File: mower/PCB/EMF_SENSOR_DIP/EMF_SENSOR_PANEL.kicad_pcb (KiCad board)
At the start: 2 copper layers, 245 x 163 mm, 360 parts, among them J1 Conn_01x03_Pin, U1 LM358

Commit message: .
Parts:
- removed the C1 at (81.6, 151.0)
- removed the C1 at (40.6, 28.0)
- removed the C1 at (245.6, 28.0)
- removed the C1 at (122.6, 110.0)
- removed the C1 at (163.6, 110.0)
- removed the C1 at (40.6, 69.0)
- removed the C1 at (163.6, 69.0)
- removed the C1 at (40.6, 151.0)
- removed the C1 at (81.6, 69.0)
- removed the C1 at (163.6, 28.0)
- removed the C1 at (204.6, 110.0)
- removed the C1 at (122.6, 151.0)
- removed the C1 at (81.6, 28.0)
- removed the C1 at (245.6, 69.0)
- removed the C1 at (122.6, 69.0)
- removed the C1 at (81.6, 110.0)
- removed the C1 at (122.6, 28.0)
- removed the C1 at (204.6, 28.0)
- removed the C1 at (204.6, 151.0)
- removed the C1 at (245.6, 151.0)
- removed the C1 at (40.6, 110.0)
- removed the C1 at (204.6, 69.0)
- removed the C1 at (163.6, 151.0)
- removed the C1 at (245.6, 110.0)
- removed the C3 at (143.8, 106.8)
- removed the C3 at (225.8, 24.8)
- removed the C3 at (266.8, 106.8)
- removed the C3 at (61.8, 24.8)
- removed the C3 at (102.8, 106.8)
- removed the C3 at (225.8, 147.8)
- removed the C3 at (143.8, 65.8)
- removed the C3 at (61.8, 147.8)
- removed the C3 at (225.8, 65.8)
- removed the C3 at (102.8, 147.8)
- removed the C3 at (184.8, 65.8)
- removed the C3 at (266.8, 65.8)
- removed the C3 at (143.8, 24.8)
- removed the C3 at (266.8, 24.8)
- removed the C3 at (225.8, 106.8)
- removed the C3 at (143.8, 147.8)
- removed the C3 at (102.8, 65.8)
- removed the C3 at (184.8, 106.8)
- removed the C3 at (266.8, 147.8)
- removed the C3 at (102.8, 24.8)
- removed the C3 at (61.8, 106.8)
- removed the C3 at (61.8, 65.8)
- removed the C3 at (184.8, 147.8)
- removed the C3 at (184.8, 24.8)
- removed the D1 at (215.1, 82.0)
- removed the D1 at (51.1, 82.0)
- removed the D1 at (256.1, 123.0)
- removed the D1 at (215.1, 41.0)
- removed the D1 at (256.1, 82.0)
- removed the D1 at (133.1, 41.0)
- removed the D1 at (133.1, 123.0)
- removed the D1 at (174.1, 82.0)
- removed the D1 at (215.1, 164.0)
- removed the D1 at (51.1, 164.0)
- removed the D1 at (215.1, 123.0)
- removed the D1 at (92.1, 164.0)
- removed the D1 at (256.1, 41.0)
- removed the D1 at (174.1, 41.0)
- removed the D1 at (133.1, 164.0)
- removed the D1 at (51.1, 41.0)
- removed the D1 at (51.1, 123.0)
- removed the D1 at (92.1, 41.0)
- removed the D1 at (133.1, 82.0)
- removed the D1 at (92.1, 123.0)
- removed the D1 at (174.1, 164.0)
- removed the D1 at (174.1, 123.0)
- removed the D1 at (256.1, 164.0)
- removed the D1 at (92.1, 82.0)
- removed the D2 at (225.7, 167.2)
- removed the D2 at (61.7, 167.2)
- removed the D2 at (266.7, 44.2)
- removed the D2 at (102.7, 44.2)
- removed the D2 at (143.7, 44.2)
- removed the D2 at (225.7, 126.2)
- removed the D2 at (184.7, 44.2)
- removed the D2 at (266.7, 85.2)
- removed the D2 at (61.7, 44.2)
- removed the D2 at (102.7, 85.2)
- removed the D2 at (61.7, 126.2)
- removed the D2 at (266.7, 126.2)
- removed the D2 at (225.7, 44.2)
- removed the D2 at (102.7, 167.2)
- removed the D2 at (61.7, 85.2)
- removed the D2 at (184.7, 126.2)
- removed the D2 at (184.7, 167.2)
- removed the D2 at (266.7, 167.2)
- removed the D2 at (143.7, 85.2)
- removed the D2 at (143.7, 167.2)
- removed the D2 at (184.7, 85.2)
- removed the D2 at (225.7, 85.2)
- removed the D2 at (143.7, 126.2)
- removed the D2 at (102.7, 126.2)
- removed the J1 at (93.4, 148.4)
- removed the J1 at (257.4, 148.4)
- removed the J1 at (175.4, 66.4)
- removed the J1 at (216.4, 66.4)
- removed the J1 at (257.4, 25.4)
- removed the J1 at (134.4, 66.4)
- removed the J1 at (257.4, 66.4)
- removed the J1 at (93.4, 107.4)
- removed the J1 at (93.4, 66.4)
- removed the J1 at (134.4, 148.4)
- removed the J1 at (216.4, 107.4)
- removed the J1 at (257.4, 107.4)
- removed the J1 at (175.4, 25.4)
- removed the J1 at (52.4, 107.4)
- removed the J1 at (175.4, 107.4)
- removed the J1 at (216.4, 25.4)
- removed the J1 at (52.4, 66.4)
- removed the J1 at (93.4, 25.4)
- removed the J1 at (52.4, 25.4)
- removed the J1 at (134.4, 107.4)
- removed the J1 at (52.4, 148.4)
- removed the J1 at (134.4, 25.4)
- removed the J1 at (175.4, 148.4)
- removed the J1 at (216.4, 148.4)
- removed the L1 at (235.4, 54.8)
- removed the L1 at (30.4, 54.8)
- removed the L1 at (71.4, 136.8)
- removed the L1 at (112.4, 136.8)
- removed the L1 at (153.4, 177.8)
- removed the L1 at (194.4, 177.8)
- removed the L1 at (30.4, 95.8)
- removed the L1 at (71.4, 95.8)
- removed the L1 at (235.4, 177.8)
- removed the L1 at (194.4, 95.8)
- removed the L1 at (30.4, 177.8)
- removed the L1 at (30.4, 136.8)
- removed the L1 at (153.4, 136.8)
- removed the L1 at (235.4, 136.8)
- removed the L1 at (153.4, 95.8)
- removed the L1 at (71.4, 54.8)
- removed the L1 at (153.4, 54.8)
- removed the L1 at (112.4, 54.8)
- removed the L1 at (112.4, 95.8)
- removed the L1 at (112.4, 177.8)
- removed the L1 at (194.4, 136.8)
- removed the L1 at (71.4, 177.8)
- removed the L1 at (235.4, 95.8)
- removed the L1 at (194.4, 54.8)
- removed the R1 at (49.9, 174.4)
- removed the R1 at (254.9, 51.4)
- removed the R1 at (172.9, 92.4)
- removed the R1 at (213.9, 174.4)
- removed the R1 at (172.9, 51.4)
- removed the R1 at (131.9, 133.4)
- removed the R1 at (90.9, 51.4)
- removed the R1 at (254.9, 133.4)
- removed the R1 at (90.9, 174.4)
- removed the R1 at (254.9, 92.4)
- removed the R1 at (172.9, 133.4)
- removed the R1 at (254.9, 174.4)
- removed the R1 at (49.9, 133.4)
- removed the R1 at (49.9, 92.4)
- removed the R1 at (90.9, 92.4)
- removed the R1 at (213.9, 51.4)
- removed the R1 at (131.9, 92.4)
- removed the R1 at (90.9, 133.4)
- removed the R1 at (49.9, 51.4)
- removed the R1 at (213.9, 133.4)
- removed the R1 at (172.9, 174.4)
- removed the R1 at (213.9, 92.4)
- removed the R1 at (131.9, 51.4)
- removed the R1 at (131.9, 174.4)
- removed the R2 at (215.3, 154.2)
- removed the R2 at (133.3, 31.2)
- removed the R2 at (51.3, 113.2)
- removed the R2 at (256.3, 72.2)
- removed the R2 at (174.3, 154.2)
- removed the R2 at (215.3, 113.2)
- removed the R2 at (215.3, 31.2)
- removed the R2 at (256.3, 31.2)
- removed the R2 at (133.3, 154.2)
- removed the R2 at (256.3, 113.2)
- removed the R2 at (92.3, 154.2)
- removed the R2 at (133.3, 113.2)
- removed the R2 at (92.3, 113.2)
- removed the R2 at (51.3, 72.2)
- removed the R2 at (256.3, 154.2)
- removed the R2 at (92.3, 72.2)
- removed the R2 at (51.3, 154.2)
- removed the R2 at (174.3, 113.2)
- removed the R2 at (215.3, 72.2)
- removed the R2 at (92.3, 31.2)
- removed the R2 at (133.3, 72.2)
- removed the R2 at (174.3, 72.2)
- removed the R2 at (51.3, 31.2)
- removed the R2 at (174.3, 31.2)
- removed the R3 at (197.2, 130.9)
- removed the R3 at (238.2, 171.9)
- removed the R3 at (197.2, 48.9)
- removed the R3 at (33.2, 130.9)
- removed the R3 at (115.2, 48.9)
- removed the R3 at (74.2, 89.9)
- removed the R3 at (115.2, 171.9)
- removed the R3 at (238.2, 89.9)
- removed the R3 at (156.2, 130.9)
- removed the R3 at (197.2, 89.9)
- removed the R3 at (33.2, 48.9)
- removed the R3 at (238.2, 130.9)
- removed the R3 at (33.2, 89.9)
- removed the R3 at (156.2, 89.9)
- removed the R3 at (115.2, 89.9)
- removed the R3 at (74.2, 171.9)
- removed the R3 at (197.2, 171.9)
- removed the R3 at (238.2, 48.9)
- removed the R3 at (74.2, 130.9)
- removed the R3 at (156.2, 171.9)
- removed the R3 at (156.2, 48.9)
- removed the R3 at (74.2, 48.9)
- removed the R3 at (115.2, 130.9)
- removed the R3 at (33.2, 171.9)
- removed the R4 at (200.6, 38.9)
- removed the R4 at (36.6, 161.9)
- removed the R4 at (36.6, 79.9)
- removed the R4 at (159.6, 161.9)
- removed the R4 at (118.6, 79.9)
- removed the R4 at (200.6, 161.9)
- removed the R4 at (36.6, 120.9)
- removed the R4 at (118.6, 38.9)
- removed the R4 at (118.6, 161.9)
- removed the R4 at (77.6, 161.9)
- removed the R4 at (36.6, 38.9)
- removed the R4 at (159.6, 79.9)
- removed the R4 at (241.6, 161.9)
- removed the R4 at (241.6, 79.9)
- removed the R4 at (200.6, 120.9)
- removed the R4 at (159.6, 120.9)
- removed the R4 at (118.6, 120.9)
- removed the R4 at (77.6, 120.9)
- removed the R4 at (200.6, 79.9)
- removed the R4 at (77.6, 38.9)
- removed the R4 at (241.6, 38.9)
- removed the R4 at (77.6, 79.9)
- removed the R4 at (159.6, 38.9)
- removed the R4 at (241.6, 120.9)
- removed the R5 at (77.2, 51.7)
- removed the R5 at (200.2, 174.7)
- removed the R5 at (159.2, 51.7)
- removed the R5 at (241.2, 174.7)
- removed the R5 at (241.2, 51.7)
- removed the R5 at (77.2, 92.7)
- removed the R5 at (118.2, 92.7)
- removed the R5 at (200.2, 51.7)
- removed the R5 at (118.2, 174.7)
- removed the R5 at (200.2, 133.7)
- removed the R5 at (118.2, 133.7)
- removed the R5 at (77.2, 133.7)
- removed the R5 at (159.2, 133.7)
- removed the R5 at (159.2, 174.7)
- removed the R5 at (200.2, 92.7)
- removed the R5 at (241.2, 133.7)
- removed the R5 at (159.2, 92.7)
- removed the R5 at (118.2, 51.7)
- removed the R5 at (36.2, 133.7)
- removed the R5 at (36.2, 51.7)
- removed the R5 at (77.2, 174.7)
- removed the R5 at (36.2, 92.7)
- removed the R5 at (241.2, 92.7)
- removed the R5 at (36.2, 174.7)
- removed the R6 at (61.9, 34.4)
- removed the R6 at (143.9, 75.4)
- removed the R6 at (102.9, 75.4)
- removed the R6 at (266.9, 75.4)
- removed the R6 at (61.9, 157.4)
- removed the R6 at (266.9, 157.4)
- removed the R6 at (266.9, 116.4)
- removed the R6 at (102.9, 157.4)
- removed the R6 at (184.9, 34.4)
- removed the R6 at (143.9, 116.4)
- removed the R6 at (61.9, 116.4)
- removed the R6 at (102.9, 116.4)
- removed the R6 at (266.9, 34.4)
- removed the R6 at (225.9, 116.4)
- removed the R6 at (225.9, 75.4)
- removed the R6 at (143.9, 34.4)
- removed the R6 at (102.9, 34.4)
- removed the R6 at (184.9, 157.4)
- removed the R6 at (184.9, 75.4)
- removed the R6 at (225.9, 34.4)
- removed the R6 at (143.9, 157.4)
- removed the R6 at (61.9, 75.4)
- removed the R6 at (225.9, 157.4)
- removed the R6 at (184.9, 116.4)
- removed the R7 at (174.7, 170.6)
- removed the R7 at (215.7, 170.6)
- removed the R7 at (51.7, 170.6)
- removed the R7 at (92.7, 47.6)
- removed the R7 at (256.7, 170.6)
- removed the R7 at (256.7, 129.6)
- removed the R7 at (215.7, 47.6)
- removed the R7 at (133.7, 47.6)
- removed the R7 at (92.7, 129.6)
- removed the R7 at (256.7, 88.6)
- removed the R7 at (51.7, 88.6)
- removed the R7 at (133.7, 88.6)
- removed the R7 at (133.7, 170.6)
- removed the R7 at (174.7, 129.6)
- removed the R7 at (256.7, 47.6)
- removed the R7 at (174.7, 88.6)
- removed the R7 at (133.7, 129.6)
- removed the R7 at (215.7, 129.6)
- removed the R7 at (215.7, 88.6)
- removed the R7 at (92.7, 88.6)
- removed the R7 at (92.7, 170.6)
- removed the R7 at (174.7, 47.6)
- removed the R7 at (51.7, 47.6)
- removed the R7 at (51.7, 129.6)
- removed the R9 at (185.0, 160.8)
- removed the R9 at (226.0, 37.8)
- removed the R9 at (144.0, 160.8)
- removed the R9 at (103.0, 37.8)
- removed the R9 at (103.0, 119.8)
- removed the R9 at (185.0, 78.8)
- removed the R9 at (144.0, 119.8)
- removed the R9 at (185.0, 119.8)
- removed the R9 at (103.0, 78.8)
- removed the R9 at (62.0, 160.8)
- removed the R9 at (267.0, 160.8)
- removed the R9 at (62.0, 119.8)
- removed the R9 at (226.0, 160.8)
- removed the R9 at (267.0, 37.8)
- removed the R9 at (62.0, 78.8)
- removed the R9 at (185.0, 37.8)
- removed the R9 at (62.0, 37.8)
- removed the R9 at (267.0, 78.8)
- removed the R9 at (144.0, 37.8)
- removed the R9 at (103.0, 160.8)
- removed the R9 at (226.0, 78.8)
- removed the R9 at (226.0, 119.8)
- removed the R9 at (144.0, 78.8)
- removed the R9 at (267.0, 119.8)
- removed the U1 at (122.2, 35.2)
- removed the U1 at (81.2, 76.2)
- removed the U1 at (81.2, 35.2)
- removed the U1 at (122.2, 117.2)
- removed the U1 at (204.2, 76.2)
- removed the U1 at (81.2, 117.2)
- removed the U1 at (122.2, 76.2)
- removed the U1 at (163.2, 35.2)
- removed the U1 at (163.2, 158.2)
- removed the U1 at (163.2, 76.2)
- removed the U1 at (163.2, 117.2)
- removed the U1 at (245.2, 35.2)
- removed the U1 at (81.2, 158.2)
- removed the U1 at (122.2, 158.2)
- removed the U1 at (204.2, 158.2)
- removed the U1 at (204.2, 117.2)
- removed the U1 at (245.2, 76.2)
- removed the U1 at (245.2, 117.2)
- removed the U1 at (204.2, 35.2)
- removed the U1 at (40.2, 117.2)
- removed the U1 at (40.2, 76.2)
- removed the U1 at (245.2, 158.2)
- removed the U1 at (40.2, 158.2)
- removed the U1 at (40.2, 35.2)
- added C1: 100nF, IMRANS_LIBRARY:C_Disc_D3.0mm_W1.6mm_P2.50mm, F.Cu at (193.3, 105.8)
- added C1: 100nF, IMRANS_LIBRARY:C_Disc_D3.0mm_W1.6mm_P2.50mm, F.Cu at (42.5, 139.8)
- added C1: 100nF, IMRANS_LIBRARY:C_Disc_D3.0mm_W1.6mm_P2.50mm, F.Cu at (117.9, 105.8)
- added C1: 100nF, IMRANS_LIBRARY:C_Disc_D3.0mm_W1.6mm_P2.50mm, F.Cu at (42.5, 71.8)
- added C1: 100nF, IMRANS_LIBRARY:C_Disc_D3.0mm_W1.6mm_P2.50mm, F.Cu at (193.3, 37.8)
- added C1: 100nF, IMRANS_LIBRARY:C_Disc_D3.0mm_W1.6mm_P2.50mm, F.Cu at (193.3, 139.8)
- added C1: 100nF, IMRANS_LIBRARY:C_Disc_D3.0mm_W1.6mm_P2.50mm, F.Cu at (117.9, 37.8)
- added C1: 100nF, IMRANS_LIBRARY:C_Disc_D3.0mm_W1.6mm_P2.50mm, F.Cu at (117.9, 139.8)
- added C1: 100nF, IMRANS_LIBRARY:C_Disc_D3.0mm_W1.6mm_P2.50mm, F.Cu at (42.5, 105.8)
- added C1: 100nF, IMRANS_LIBRARY:C_Disc_D3.0mm_W1.6mm_P2.50mm, F.Cu at (117.9, 71.8)
- added C1: 100nF, IMRANS_LIBRARY:C_Disc_D3.0mm_W1.6mm_P2.50mm, F.Cu at (42.5, 37.8)
- added C1: 100nF, IMRANS_LIBRARY:C_Disc_D3.0mm_W1.6mm_P2.50mm, F.Cu at (193.3, 71.8)
- added C2: 10uF, IMRANS_LIBRARY:C_Disc_D3.0mm_W1.6mm_P2.50mm, F.Cu at (245.9, 149.2)
- added C2: 10uF, IMRANS_LIBRARY:C_Disc_D3.0mm_W1.6mm_P2.50mm, F.Cu at (170.5, 47.2)
- added C2: 10uF, IMRANS_LIBRARY:C_Disc_D3.0mm_W1.6mm_P2.50mm, F.Cu at (170.5, 149.2)
- added C2: 10uF, IMRANS_LIBRARY:C_Disc_D3.0mm_W1.6mm_P2.50mm, F.Cu at (170.5, 81.2)
- added C2: 10uF, IMRANS_LIBRARY:C_Disc_D3.0mm_W1.6mm_P2.50mm, F.Cu at (245.9, 47.2)
- added C2: 10uF, IMRANS_LIBRARY:C_Disc_D3.0mm_W1.6mm_P2.50mm, F.Cu at (245.9, 115.2)
- added C2: 10uF, IMRANS_LIBRARY:C_Disc_D3.0mm_W1.6mm_P2.50mm, F.Cu at (95.1, 47.2)
- added C2: 10uF, IMRANS_LIBRARY:C_Disc_D3.0mm_W1.6mm_P2.50mm, F.Cu at (170.5, 115.2)
- added C2: 10uF, IMRANS_LIBRARY:C_Disc_D3.0mm_W1.6mm_P2.50mm, F.Cu at (95.1, 115.2)
- added C2: 10uF, IMRANS_LIBRARY:C_Disc_D3.0mm_W1.6mm_P2.50mm, F.Cu at (245.9, 81.2)
- added C2: 10uF, IMRANS_LIBRARY:C_Disc_D3.0mm_W1.6mm_P2.50mm, F.Cu at (95.1, 149.2)
- added C2: 10uF, IMRANS_LIBRARY:C_Disc_D3.0mm_W1.6mm_P2.50mm, F.Cu at (95.1, 81.2)
- added C3: 100nF (104), IMRANS_LIBRARY:C_Disc_D3.0mm_W1.6mm_P2.50mm, F.Cu at (83.1, 43.8)
- added C3: 100nF (104), IMRANS_LIBRARY:C_Disc_D3.0mm_W1.6mm_P2.50mm, F.Cu at (233.9, 43.8)
- added C3: 100nF (104), IMRANS_LIBRARY:C_Disc_D3.0mm_W1.6mm_P2.50mm, F.Cu at (158.5, 145.8)
- added C3: 100nF (104), IMRANS_LIBRARY:C_Disc_D3.0mm_W1.6mm_P2.50mm, F.Cu at (83.1, 77.8)
- added C3: 100nF (104), IMRANS_LIBRARY:C_Disc_D3.0mm_W1.6mm_P2.50mm, F.Cu at (83.1, 111.8)
- added C3: 100nF (104), IMRANS_LIBRARY:C_Disc_D3.0mm_W1.6mm_P2.50mm, F.Cu at (158.5, 43.8)
- added C3: 100nF (104), IMRANS_LIBRARY:C_Disc_D3.0mm_W1.6mm_P2.50mm, F.Cu at (233.9, 77.8)
- added C3: 100nF (104), IMRANS_LIBRARY:C_Disc_D3.0mm_W1.6mm_P2.50mm, F.Cu at (158.5, 77.8)
- added C3: 100nF (104), IMRANS_LIBRARY:C_Disc_D3.0mm_W1.6mm_P2.50mm, F.Cu at (233.9, 111.8)
- added C3: 100nF (104), IMRANS_LIBRARY:C_Disc_D3.0mm_W1.6mm_P2.50mm, F.Cu at (233.9, 145.8)
- added C3: 100nF (104), IMRANS_LIBRARY:C_Disc_D3.0mm_W1.6mm_P2.50mm, F.Cu at (158.5, 111.8)
- added C3: 100nF (104), IMRANS_LIBRARY:C_Disc_D3.0mm_W1.6mm_P2.50mm, F.Cu at (83.1, 145.8)
- added C4: 10uF, IMRANS_LIBRARY:C_Disc_D3.0mm_W1.6mm_P2.50mm, F.Cu at (177.1, 60.4)
- added C4: 10uF, IMRANS_LIBRARY:C_Disc_D3.0mm_W1.6mm_P2.50mm, F.Cu at (101.7, 94.4)
- added C4: 10uF, IMRANS_LIBRARY:C_Disc_D3.0mm_W1.6mm_P2.50mm, F.Cu at (252.5, 26.4)
- added C4: 10uF, IMRANS_LIBRARY:C_Disc_D3.0mm_W1.6mm_P2.50mm, F.Cu at (252.5, 128.4)
- added C4: 10uF, IMRANS_LIBRARY:C_Disc_D3.0mm_W1.6mm_P2.50mm, F.Cu at (252.5, 94.4)
- added C4: 10uF, IMRANS_LIBRARY:C_Disc_D3.0mm_W1.6mm_P2.50mm, F.Cu at (101.7, 26.4)
- added C4: 10uF, IMRANS_LIBRARY:C_Disc_D3.0mm_W1.6mm_P2.50mm, F.Cu at (177.1, 128.4)
- added C4: 10uF, IMRANS_LIBRARY:C_Disc_D3.0mm_W1.6mm_P2.50mm, F.Cu at (177.1, 94.4)
- added C4: 10uF, IMRANS_LIBRARY:C_Disc_D3.0mm_W1.6mm_P2.50mm, F.Cu at (101.7, 128.4)
- added C4: 10uF, IMRANS_LIBRARY:C_Disc_D3.0mm_W1.6mm_P2.50mm, F.Cu at (101.7, 60.4)
- added C4: 10uF, IMRANS_LIBRARY:C_Disc_D3.0mm_W1.6mm_P2.50mm, F.Cu at (252.5, 60.4)
- added C4: 10uF, IMRANS_LIBRARY:C_Disc_D3.0mm_W1.6mm_P2.50mm, F.Cu at (177.1, 26.4)
- added C5: 1nF, IMRANS_LIBRARY:C_Disc_D3.0mm_W1.6mm_P2.50mm, F.Cu at (45.3, 29.8)
- added C5: 1nF, IMRANS_LIBRARY:C_Disc_D3.0mm_W1.6mm_P2.50mm, F.Cu at (45.3, 63.8)
- added C5: 1nF, IMRANS_LIBRARY:C_Disc_D3.0mm_W1.6mm_P2.50mm, F.Cu at (196.1, 131.8)
- added C5: 1nF, IMRANS_LIBRARY:C_Disc_D3.0mm_W1.6mm_P2.50mm, F.Cu at (120.7, 29.8)
- added C5: 1nF, IMRANS_LIBRARY:C_Disc_D3.0mm_W1.6mm_P2.50mm, F.Cu at (120.7, 97.8)
- added C5: 1nF, IMRANS_LIBRARY:C_Disc_D3.0mm_W1.6mm_P2.50mm, F.Cu at (45.3, 131.8)
- added C5: 1nF, IMRANS_LIBRARY:C_Disc_D3.0mm_W1.6mm_P2.50mm, F.Cu at (196.1, 97.8)
- added C5: 1nF, IMRANS_LIBRARY:C_Disc_D3.0mm_W1.6mm_P2.50mm, F.Cu at (196.1, 29.8)
- added C5: 1nF, IMRANS_LIBRARY:C_Disc_D3.0mm_W1.6mm_P2.50mm, F.Cu at (196.1, 63.8)
- added C5: 1nF, IMRANS_LIBRARY:C_Disc_D3.0mm_W1.6mm_P2.50mm, F.Cu at (120.7, 63.8)
- added C5: 1nF, IMRANS_LIBRARY:C_Disc_D3.0mm_W1.6mm_P2.50mm, F.Cu at (120.7, 131.8)
- added C5: 1nF, IMRANS_LIBRARY:C_Disc_D3.0mm_W1.6mm_P2.50mm, F.Cu at (45.3, 97.8)
- added C6: 0.01uF, IMRANS_LIBRARY:C_Disc_D3.0mm_W1.6mm_P2.50mm, F.Cu at (194.9, 125.2)
- added C6: 0.01uF, IMRANS_LIBRARY:C_Disc_D3.0mm_W1.6mm_P2.50mm, F.Cu at (194.9, 57.2)
- added C6: 0.01uF, IMRANS_LIBRARY:C_Disc_D3.0mm_W1.6mm_P2.50mm, F.Cu at (44.1, 91.2)
- added C6: 0.01uF, IMRANS_LIBRARY:C_Disc_D3.0mm_W1.6mm_P2.50mm, F.Cu at (194.9, 91.2)
- added C6: 0.01uF, IMRANS_LIBRARY:C_Disc_D3.0mm_W1.6mm_P2.50mm, F.Cu at (119.5, 125.2)
- added C6: 0.01uF, IMRANS_LIBRARY:C_Disc_D3.0mm_W1.6mm_P2.50mm, F.Cu at (119.5, 91.2)
- added C6: 0.01uF, IMRANS_LIBRARY:C_Disc_D3.0mm_W1.6mm_P2.50mm, F.Cu at (44.1, 57.2)
- added C6: 0.01uF, IMRANS_LIBRARY:C_Disc_D3.0mm_W1.6mm_P2.50mm, F.Cu at (119.5, 57.2)
- added C6: 0.01uF, IMRANS_LIBRARY:C_Disc_D3.0mm_W1.6mm_P2.50mm, F.Cu at (194.9, 23.2)
- added C6: 0.01uF, IMRANS_LIBRARY:C_Disc_D3.0mm_W1.6mm_P2.50mm, F.Cu at (44.1, 125.2)
- added C6: 0.01uF, IMRANS_LIBRARY:C_Disc_D3.0mm_W1.6mm_P2.50mm, F.Cu at (44.1, 23.2)
- added C6: 0.01uF, IMRANS_LIBRARY:C_Disc_D3.0mm_W1.6mm_P2.50mm, F.Cu at (119.5, 23.2)
- added D1: 1N4007, IMRANS_LIBRARY:R_Axial_DIN0207_L6.3mm_D2.5mm_P10.16mm_Horizontal_2, F.Cu at (159.2, 74.8)
- added D1: 1N4007, IMRANS_LIBRARY:R_Axial_DIN0207_L6.3mm_D2.5mm_P10.16mm_Horizontal_2, F.Cu at (83.8, 142.8)
- added D1: 1N4007, IMRANS_LIBRARY:R_Axial_DIN0207_L6.3mm_D2.5mm_P10.16mm_Horizontal_2, F.Cu at (159.2, 108.8)
- added D1: 1N4007, IMRANS_LIBRARY:R_Axial_DIN0207_L6.3mm_D2.5mm_P10.16mm_Horizontal_2, F.Cu at (83.8, 40.8)
- added D1: 1N4007, IMRANS_LIBRARY:R_Axial_DIN0207_L6.3mm_D2.5mm_P10.16mm_Horizontal_2, F.Cu at (83.8, 74.8)
- added D1: 1N4007, IMRANS_LIBRARY:R_Axial_DIN0207_L6.3mm_D2.5mm_P10.16mm_Horizontal_2, F.Cu at (159.2, 142.8)
- added D1: 1N4007, IMRANS_LIBRARY:R_Axial_DIN0207_L6.3mm_D2.5mm_P10.16mm_Horizontal_2, F.Cu at (234.6, 40.8)
- added D1: 1N4007, IMRANS_LIBRARY:R_Axial_DIN0207_L6.3mm_D2.5mm_P10.16mm_Horizontal_2, F.Cu at (83.8, 108.8)
- added D1: 1N4007, IMRANS_LIBRARY:R_Axial_DIN0207_L6.3mm_D2.5mm_P10.16mm_Horizontal_2, F.Cu at (234.6, 142.8)
- added D1: 1N4007, IMRANS_LIBRARY:R_Axial_DIN0207_L6.3mm_D2.5mm_P10.16mm_Horizontal_2, F.Cu at (159.2, 40.8)
- added D1: 1N4007, IMRANS_LIBRARY:R_Axial_DIN0207_L6.3mm_D2.5mm_P10.16mm_Horizontal_2, F.Cu at (234.6, 108.8)
- added D1: 1N4007, IMRANS_LIBRARY:R_Axial_DIN0207_L6.3mm_D2.5mm_P10.16mm_Horizontal_2, F.Cu at (234.6, 74.8)
- added D2: 1N5819, IMRANS_LIBRARY:R_Axial_DIN0207_L6.3mm_D2.5mm_P10.16mm_Horizontal_2, F.Cu at (223.8, 101.4)
- added D2: 1N5819, IMRANS_LIBRARY:R_Axial_DIN0207_L6.3mm_D2.5mm_P10.16mm_Horizontal_2, F.Cu at (148.4, 101.4)
- added D2: 1N5819, IMRANS_LIBRARY:R_Axial_DIN0207_L6.3mm_D2.5mm_P10.16mm_Horizontal_2, F.Cu at (73.0, 101.4)
- added D2: 1N5819, IMRANS_LIBRARY:R_Axial_DIN0207_L6.3mm_D2.5mm_P10.16mm_Horizontal_2, F.Cu at (223.8, 33.4)
- added D2: 1N5819, IMRANS_LIBRARY:R_Axial_DIN0207_L6.3mm_D2.5mm_P10.16mm_Horizontal_2, F.Cu at (223.8, 135.4)
- added D2: 1N5819, IMRANS_LIBRARY:R_Axial_DIN0207_L6.3mm_D2.5mm_P10.16mm_Horizontal_2, F.Cu at (73.0, 33.4)
- added D2: 1N5819, IMRANS_LIBRARY:R_Axial_DIN0207_L6.3mm_D2.5mm_P10.16mm_Horizontal_2, F.Cu at (148.4, 135.4)
- added D2: 1N5819, IMRANS_LIBRARY:R_Axial_DIN0207_L6.3mm_D2.5mm_P10.16mm_Horizontal_2, F.Cu at (223.8, 67.4)
- added D2: 1N5819, IMRANS_LIBRARY:R_Axial_DIN0207_L6.3mm_D2.5mm_P10.16mm_Horizontal_2, F.Cu at (148.4, 33.4)
- added D2: 1N5819, IMRANS_LIBRARY:R_Axial_DIN0207_L6.3mm_D2.5mm_P10.16mm_Horizontal_2, F.Cu at (73.0, 135.4)
- added D2: 1N5819, IMRANS_LIBRARY:R_Axial_DIN0207_L6.3mm_D2.5mm_P10.16mm_Horizontal_2, F.Cu at (148.4, 67.4)
- added D2: 1N5819, IMRANS_LIBRARY:R_Axial_DIN0207_L6.3mm_D2.5mm_P10.16mm_Horizontal_2, F.Cu at (73.0, 67.4)
- added J1: Conn_01x03_Pin, IMRANS_LIBRARY:PinHeader_1x03_P2.54mm_Vertical, F.Cu at (166.9, 61.4)
- added J1: Conn_01x03_Pin, IMRANS_LIBRARY:PinHeader_1x03_P2.54mm_Vertical, F.Cu at (166.9, 129.4)
- added J1: Conn_01x03_Pin, IMRANS_LIBRARY:PinHeader_1x03_P2.54mm_Vertical, F.Cu at (242.3, 27.4)
- added J1: Conn_01x03_Pin, IMRANS_LIBRARY:PinHeader_1x03_P2.54mm_Vertical, F.Cu at (242.3, 129.4)
- added J1: Conn_01x03_Pin, IMRANS_LIBRARY:PinHeader_1x03_P2.54mm_Vertical, F.Cu at (242.3, 61.4)
- added J1: Conn_01x03_Pin, IMRANS_LIBRARY:PinHeader_1x03_P2.54mm_Vertical, F.Cu at (91.5, 27.4)
- added J1: Conn_01x03_Pin, IMRANS_LIBRARY:PinHeader_1x03_P2.54mm_Vertical, F.Cu at (166.9, 95.4)
- added J1: Conn_01x03_Pin, IMRANS_LIBRARY:PinHeader_1x03_P2.54mm_Vertical, F.Cu at (166.9, 27.4)
- added J1: Conn_01x03_Pin, IMRANS_LIBRARY:PinHeader_1x03_P2.54mm_Vertical, F.Cu at (91.5, 129.4)
- added J1: Conn_01x03_Pin, IMRANS_LIBRARY:PinHeader_1x03_P2.54mm_Vertical, F.Cu at (91.5, 61.4)
- added J1: Conn_01x03_Pin, IMRANS_LIBRARY:PinHeader_1x03_P2.54mm_Vertical, F.Cu at (242.3, 95.4)
- added J1: Conn_01x03_Pin, IMRANS_LIBRARY:PinHeader_1x03_P2.54mm_Vertical, F.Cu at (91.5, 95.4)
- added L1: L, Inductor_THT:L_Radial_D10.0mm_P5.00mm_Fastron_07M, F.Cu at (191.1, 112.4)
- added L1: L, Inductor_THT:L_Radial_D10.0mm_P5.00mm_Fastron_07M, F.Cu at (115.7, 44.4)
- added L1: L, Inductor_THT:L_Radial_D10.0mm_P5.00mm_Fastron_07M, F.Cu at (115.7, 78.4)
- added L1: L, Inductor_THT:L_Radial_D10.0mm_P5.00mm_Fastron_07M, F.Cu at (115.7, 146.4)
- added L1: L, Inductor_THT:L_Radial_D10.0mm_P5.00mm_Fastron_07M, F.Cu at (191.1, 44.4)
- added L1: L, Inductor_THT:L_Radial_D10.0mm_P5.00mm_Fastron_07M, F.Cu at (40.3, 44.4)
- added L1: L, Inductor_THT:L_Radial_D10.0mm_P5.00mm_Fastron_07M, F.Cu at (191.1, 78.4)
- added L1: L, Inductor_THT:L_Radial_D10.0mm_P5.00mm_Fastron_07M, F.Cu at (40.3, 78.4)
- added L1: L, Inductor_THT:L_Radial_D10.0mm_P5.00mm_Fastron_07M, F.Cu at (40.3, 112.4)
- added L1: L, Inductor_THT:L_Radial_D10.0mm_P5.00mm_Fastron_07M, F.Cu at (40.3, 146.4)
- added L1: L, Inductor_THT:L_Radial_D10.0mm_P5.00mm_Fastron_07M, F.Cu at (115.7, 112.4)
- added L1: L, Inductor_THT:L_Radial_D10.0mm_P5.00mm_Fastron_07M, F.Cu at (191.1, 146.4)
- added R1: 10k, IMRANS_LIBRARY:R_Axial_DIN0207_L6.3mm_D2.5mm_P10.16mm_Horizontal_2, F.Cu at (197.9, 82.4)
- added R1: 10k, IMRANS_LIBRARY:R_Axial_DIN0207_L6.3mm_D2.5mm_P10.16mm_Horizontal_2, F.Cu at (197.9, 116.4)
- added R1: 10k, IMRANS_LIBRARY:R_Axial_DIN0207_L6.3mm_D2.5mm_P10.16mm_Horizontal_2, F.Cu at (197.9, 48.4)
- added R1: 10k, IMRANS_LIBRARY:R_Axial_DIN0207_L6.3mm_D2.5mm_P10.16mm_Horizontal_2, F.Cu at (122.5, 48.4)
- added R1: 10k, IMRANS_LIBRARY:R_Axial_DIN0207_L6.3mm_D2.5mm_P10.16mm_Horizontal_2, F.Cu at (47.1, 116.4)
- added R1: 10k, IMRANS_LIBRARY:R_Axial_DIN0207_L6.3mm_D2.5mm_P10.16mm_Horizontal_2, F.Cu at (47.1, 150.4)
- added R1: 10k, IMRANS_LIBRARY:R_Axial_DIN0207_L6.3mm_D2.5mm_P10.16mm_Horizontal_2, F.Cu at (122.5, 150.4)
- added R1: 10k, IMRANS_LIBRARY:R_Axial_DIN0207_L6.3mm_D2.5mm_P10.16mm_Horizontal_2, F.Cu at (122.5, 116.4)
- added R1: 10k, IMRANS_LIBRARY:R_Axial_DIN0207_L6.3mm_D2.5mm_P10.16mm_Horizontal_2, F.Cu at (47.1, 82.4)
- added R1: 10k, IMRANS_LIBRARY:R_Axial_DIN0207_L6.3mm_D2.5mm_P10.16mm_Horizontal_2, F.Cu at (197.9, 150.4)
- added R1: 10k, IMRANS_LIBRARY:R_Axial_DIN0207_L6.3mm_D2.5mm_P10.16mm_Horizontal_2, F.Cu at (47.1, 48.4)
- added R1: 10k, IMRANS_LIBRARY:R_Axial_DIN0207_L6.3mm_D2.5mm_P10.16mm_Horizontal_2, F.Cu at (122.5, 82.4)
- added R10: 10K, IMRANS_LIBRARY:R_Axial_DIN0207_L6.3mm_D2.5mm_P10.16mm_Horizontal_2, F.Cu at (67.1, 49.7)
- added R10: 10K, IMRANS_LIBRARY:R_Axial_DIN0207_L6.3mm_D2.5mm_P10.16mm_Horizontal_2, F.Cu at (217.9, 151.7)
- added R10: 10K, IMRANS_LIBRARY:R_Axial_DIN0207_L6.3mm_D2.5mm_P10.16mm_Horizontal_2, F.Cu at (67.1, 151.7)
- added R10: 10K, IMRANS_LIBRARY:R_Axial_DIN0207_L6.3mm_D2.5mm_P10.16mm_Horizontal_2, F.Cu at (217.9, 83.7)
- added R10: 10K, IMRANS_LIBRARY:R_Axial_DIN0207_L6.3mm_D2.5mm_P10.16mm_Horizontal_2, F.Cu at (142.5, 49.7)
- added R10: 10K, IMRANS_LIBRARY:R_Axial_DIN0207_L6.3mm_D2.5mm_P10.16mm_Horizontal_2, F.Cu at (142.5, 83.7)
- added R10: 10K, IMRANS_LIBRARY:R_Axial_DIN0207_L6.3mm_D2.5mm_P10.16mm_Horizontal_2, F.Cu at (217.9, 117.7)
- added R10: 10K, IMRANS_LIBRARY:R_Axial_DIN0207_L6.3mm_D2.5mm_P10.16mm_Horizontal_2, F.Cu at (217.9, 49.7)
- added R10: 10K, IMRANS_LIBRARY:R_Axial_DIN0207_L6.3mm_D2.5mm_P10.16mm_Horizontal_2, F.Cu at (142.5, 117.7)
- added R10: 10K, IMRANS_LIBRARY:R_Axial_DIN0207_L6.3mm_D2.5mm_P10.16mm_Horizontal_2, F.Cu at (67.1, 83.7)
- added R10: 10K, IMRANS_LIBRARY:R_Axial_DIN0207_L6.3mm_D2.5mm_P10.16mm_Horizontal_2, F.Cu at (142.5, 151.7)
- added R10: 10K, IMRANS_LIBRARY:R_Axial_DIN0207_L6.3mm_D2.5mm_P10.16mm_Horizontal_2, F.Cu at (67.1, 117.7)
- added R11: 10K, IMRANS_LIBRARY:R_Axial_DIN0207_L6.3mm_D2.5mm_P10.16mm_Horizontal_2, F.Cu at (65.7, 128.8)
- added R11: 10K, IMRANS_LIBRARY:R_Axial_DIN0207_L6.3mm_D2.5mm_P10.16mm_Horizontal_2, F.Cu at (65.7, 94.8)
- added R11: 10K, IMRANS_LIBRARY:R_Axial_DIN0207_L6.3mm_D2.5mm_P10.16mm_Horizontal_2, F.Cu at (216.5, 94.8)
- added R11: 10K, IMRANS_LIBRARY:R_Axial_DIN0207_L6.3mm_D2.5mm_P10.16mm_Horizontal_2, F.Cu at (141.1, 60.8)
- added R11: 10K, IMRANS_LIBRARY:R_Axial_DIN0207_L6.3mm_D2.5mm_P10.16mm_Horizontal_2, F.Cu at (65.7, 60.8)
- added R11: 10K, IMRANS_LIBRARY:R_Axial_DIN0207_L6.3mm_D2.5mm_P10.16mm_Horizontal_2, F.Cu at (141.1, 128.8)
- added R11: 10K, IMRANS_LIBRARY:R_Axial_DIN0207_L6.3mm_D2.5mm_P10.16mm_Horizontal_2, F.Cu at (216.5, 26.8)
- added R11: 10K, IMRANS_LIBRARY:R_Axial_DIN0207_L6.3mm_D2.5mm_P10.16mm_Horizontal_2, F.Cu at (141.1, 26.8)
- added R11: 10K, IMRANS_LIBRARY:R_Axial_DIN0207_L6.3mm_D2.5mm_P10.16mm_Horizontal_2, F.Cu at (216.5, 60.8)
- added R11: 10K, IMRANS_LIBRARY:R_Axial_DIN0207_L6.3mm_D2.5mm_P10.16mm_Horizontal_2, F.Cu at (65.7, 26.8)
- added R11: 10K, IMRANS_LIBRARY:R_Axial_DIN0207_L6.3mm_D2.5mm_P10.16mm_Horizontal_2, F.Cu at (141.1, 94.8)
- added R11: 10K, IMRANS_LIBRARY:R_Axial_DIN0207_L6.3mm_D2.5mm_P10.16mm_Horizontal_2, F.Cu at (216.5, 128.8)
- added R12: 100K, IMRANS_LIBRARY:R_Axial_DIN0207_L6.3mm_D2.5mm_P10.16mm_Horizontal_2, F.Cu at (239.2, 32.2)
- added R12: 100K, IMRANS_LIBRARY:R_Axial_DIN0207_L6.3mm_D2.5mm_P10.16mm_Horizontal_2, F.Cu at (163.8, 100.2)
- added R12: 100K, IMRANS_LIBRARY:R_Axial_DIN0207_L6.3mm_D2.5mm_P10.16mm_Horizontal_2, F.Cu at (163.8, 32.2)
- added R12: 100K, IMRANS_LIBRARY:R_Axial_DIN0207_L6.3mm_D2.5mm_P10.16mm_Horizontal_2, F.Cu at (239.2, 66.2)
- added R12: 100K, IMRANS_LIBRARY:R_Axial_DIN0207_L6.3mm_D2.5mm_P10.16mm_Horizontal_2, F.Cu at (88.4, 66.2)
- added R12: 100K, IMRANS_LIBRARY:R_Axial_DIN0207_L6.3mm_D2.5mm_P10.16mm_Horizontal_2, F.Cu at (163.8, 66.2)
- added R12: 100K, IMRANS_LIBRARY:R_Axial_DIN0207_L6.3mm_D2.5mm_P10.16mm_Horizontal_2, F.Cu at (88.4, 100.2)
- added R12: 100K, IMRANS_LIBRARY:R_Axial_DIN0207_L6.3mm_D2.5mm_P10.16mm_Horizontal_2, F.Cu at (239.2, 100.2)
- added R12: 100K, IMRANS_LIBRARY:R_Axial_DIN0207_L6.3mm_D2.5mm_P10.16mm_Horizontal_2, F.Cu at (163.8, 134.2)
- added R12: 100K, IMRANS_LIBRARY:R_Axial_DIN0207_L6.3mm_D2.5mm_P10.16mm_Horizontal_2, F.Cu at (239.2, 134.2)
- added R12: 100K, IMRANS_LIBRARY:R_Axial_DIN0207_L6.3mm_D2.5mm_P10.16mm_Horizontal_2, F.Cu at (88.4, 134.2)
- added R12: 100K, IMRANS_LIBRARY:R_Axial_DIN0207_L6.3mm_D2.5mm_P10.16mm_Horizontal_2, F.Cu at (88.4, 32.2)
- added R2: 10k, IMRANS_LIBRARY:R_Axial_DIN0207_L6.3mm_D2.5mm_P10.16mm_Horizontal_2, F.Cu at (223.8, 26.8)
- added R2: 10k, IMRANS_LIBRARY:R_Axial_DIN0207_L6.3mm_D2.5mm_P10.16mm_Horizontal_2, F.Cu at (73.0, 94.8)
- added R2: 10k, IMRANS_LIBRARY:R_Axial_DIN0207_L6.3mm_D2.5mm_P10.16mm_Horizontal_2, F.Cu at (148.4, 60.8)
- added R2: 10k, IMRANS_LIBRARY:R_Axial_DIN0207_L6.3mm_D2.5mm_P10.16mm_Horizontal_2, F.Cu at (148.4, 128.8)
- added R2: 10k, IMRANS_LIBRARY:R_Axial_DIN0207_L6.3mm_D2.5mm_P10.16mm_Horizontal_2, F.Cu at (148.4, 26.8)
- added R2: 10k, IMRANS_LIBRARY:R_Axial_DIN0207_L6.3mm_D2.5mm_P10.16mm_Horizontal_2, F.Cu at (73.0, 60.8)
- added R2: 10k, IMRANS_LIBRARY:R_Axial_DIN0207_L6.3mm_D2.5mm_P10.16mm_Horizontal_2, F.Cu at (223.8, 128.8)
- added R2: 10k, IMRANS_LIBRARY:R_Axial_DIN0207_L6.3mm_D2.5mm_P10.16mm_Horizontal_2, F.Cu at (223.8, 60.8)
- added R2: 10k, IMRANS_LIBRARY:R_Axial_DIN0207_L6.3mm_D2.5mm_P10.16mm_Horizontal_2, F.Cu at (73.0, 26.8)
- added R2: 10k, IMRANS_LIBRARY:R_Axial_DIN0207_L6.3mm_D2.5mm_P10.16mm_Horizontal_2, F.Cu at (223.8, 94.8)
- added R2: 10k, IMRANS_LIBRARY:R_Axial_DIN0207_L6.3mm_D2.5mm_P10.16mm_Horizontal_2, F.Cu at (73.0, 128.8)
- added R2: 10k, IMRANS_LIBRARY:R_Axial_DIN0207_L6.3mm_D2.5mm_P10.16mm_Horizontal_2, F.Cu at (148.4, 94.8)
- added R3: 220, IMRANS_LIBRARY:R_Axial_DIN0207_L6.3mm_D2.5mm_P10.16mm_Horizontal_2, F.Cu at (39.7, 139.1)
- added R3: 220, IMRANS_LIBRARY:R_Axial_DIN0207_L6.3mm_D2.5mm_P10.16mm_Horizontal_2, F.Cu at (190.5, 139.1)
- added R3: 220, IMRANS_LIBRARY:R_Axial_DIN0207_L6.3mm_D2.5mm_P10.16mm_Horizontal_2, F.Cu at (115.1, 37.1)
- added R3: 220, IMRANS_LIBRARY:R_Axial_DIN0207_L6.3mm_D2.5mm_P10.16mm_Horizontal_2, F.Cu at (190.5, 105.1)
- added R3: 220, IMRANS_LIBRARY:R_Axial_DIN0207_L6.3mm_D2.5mm_P10.16mm_Horizontal_2, F.Cu at (39.7, 37.1)
- added R3: 220, IMRANS_LIBRARY:R_Axial_DIN0207_L6.3mm_D2.5mm_P10.16mm_Horizontal_2, F.Cu at (190.5, 37.1)
- added R3: 220, IMRANS_LIBRARY:R_Axial_DIN0207_L6.3mm_D2.5mm_P10.16mm_Horizontal_2, F.Cu at (39.7, 71.1)
- added R3: 220, IMRANS_LIBRARY:R_Axial_DIN0207_L6.3mm_D2.5mm_P10.16mm_Horizontal_2, F.Cu at (115.1, 139.1)
- added R3: 220, IMRANS_LIBRARY:R_Axial_DIN0207_L6.3mm_D2.5mm_P10.16mm_Horizontal_2, F.Cu at (39.7, 105.1)
- added R3: 220, IMRANS_LIBRARY:R_Axial_DIN0207_L6.3mm_D2.5mm_P10.16mm_Horizontal_2, F.Cu at (115.1, 105.1)
- added R3: 220, IMRANS_LIBRARY:R_Axial_DIN0207_L6.3mm_D2.5mm_P10.16mm_Horizontal_2, F.Cu at (190.5, 71.1)
- added R3: 220, IMRANS_LIBRARY:R_Axial_DIN0207_L6.3mm_D2.5mm_P10.16mm_Horizontal_2, F.Cu at (115.1, 71.1)
- added R4: 1M, IMRANS_LIBRARY:R_Axial_DIN0207_L6.3mm_D2.5mm_P10.16mm_Horizontal_2, F.Cu at (51.9, 138.1)
- added R4: 1M, IMRANS_LIBRARY:R_Axial_DIN0207_L6.3mm_D2.5mm_P10.16mm_Horizontal_2, F.Cu at (202.7, 70.1)
- added R4: 1M, IMRANS_LIBRARY:R_Axial_DIN0207_L6.3mm_D2.5mm_P10.16mm_Horizontal_2, F.Cu at (127.3, 70.1)
- added R4: 1M, IMRANS_LIBRARY:R_Axial_DIN0207_L6.3mm_D2.5mm_P10.16mm_Horizontal_2, F.Cu at (127.3, 104.1)
- added R4: 1M, IMRANS_LIBRARY:R_Axial_DIN0207_L6.3mm_D2.5mm_P10.16mm_Horizontal_2, F.Cu at (127.3, 138.1)
- added R4: 1M, IMRANS_LIBRARY:R_Axial_DIN0207_L6.3mm_D2.5mm_P10.16mm_Horizontal_2, F.Cu at (51.9, 104.1)
- added R4: 1M, IMRANS_LIBRARY:R_Axial_DIN0207_L6.3mm_D2.5mm_P10.16mm_Horizontal_2, F.Cu at (202.7, 138.1)
- added R4: 1M, IMRANS_LIBRARY:R_Axial_DIN0207_L6.3mm_D2.5mm_P10.16mm_Horizontal_2, F.Cu at (202.7, 104.1)
- added R4: 1M, IMRANS_LIBRARY:R_Axial_DIN0207_L6.3mm_D2.5mm_P10.16mm_Horizontal_2, F.Cu at (51.9, 36.1)
- added R4: 1M, IMRANS_LIBRARY:R_Axial_DIN0207_L6.3mm_D2.5mm_P10.16mm_Horizontal_2, F.Cu at (127.3, 36.1)
- added R4: 1M, IMRANS_LIBRARY:R_Axial_DIN0207_L6.3mm_D2.5mm_P10.16mm_Horizontal_2, F.Cu at (51.9, 70.1)
- added R4: 1M, IMRANS_LIBRARY:R_Axial_DIN0207_L6.3mm_D2.5mm_P10.16mm_Horizontal_2, F.Cu at (202.7, 36.1)
- added R5: 1K, IMRANS_LIBRARY:R_Axial_DIN0207_L6.3mm_D2.5mm_P10.16mm_Horizontal_2, F.Cu at (123.9, 110.3)
- added R5: 1K, IMRANS_LIBRARY:R_Axial_DIN0207_L6.3mm_D2.5mm_P10.16mm_Horizontal_2, F.Cu at (199.3, 42.3)
- added R5: 1K, IMRANS_LIBRARY:R_Axial_DIN0207_L6.3mm_D2.5mm_P10.16mm_Horizontal_2, F.Cu at (123.9, 42.3)
- added R5: 1K, IMRANS_LIBRARY:R_Axial_DIN0207_L6.3mm_D2.5mm_P10.16mm_Horizontal_2, F.Cu at (48.5, 42.3)
- added R5: 1K, IMRANS_LIBRARY:R_Axial_DIN0207_L6.3mm_D2.5mm_P10.16mm_Horizontal_2, F.Cu at (123.9, 76.3)
- added R5: 1K, IMRANS_LIBRARY:R_Axial_DIN0207_L6.3mm_D2.5mm_P10.16mm_Horizontal_2, F.Cu at (199.3, 144.3)
- added R5: 1K, IMRANS_LIBRARY:R_Axial_DIN0207_L6.3mm_D2.5mm_P10.16mm_Horizontal_2, F.Cu at (123.9, 144.3)
- added R5: 1K, IMRANS_LIBRARY:R_Axial_DIN0207_L6.3mm_D2.5mm_P10.16mm_Horizontal_2, F.Cu at (48.5, 144.3)
- added R5: 1K, IMRANS_LIBRARY:R_Axial_DIN0207_L6.3mm_D2.5mm_P10.16mm_Horizontal_2, F.Cu at (199.3, 110.3)
- added R5: 1K, IMRANS_LIBRARY:R_Axial_DIN0207_L6.3mm_D2.5mm_P10.16mm_Horizontal_2, F.Cu at (48.5, 110.3)
- added R5: 1K, IMRANS_LIBRARY:R_Axial_DIN0207_L6.3mm_D2.5mm_P10.16mm_Horizontal_2, F.Cu at (199.3, 76.3)
- added R5: 1K, IMRANS_LIBRARY:R_Axial_DIN0207_L6.3mm_D2.5mm_P10.16mm_Horizontal_2, F.Cu at (48.5, 76.3)
- added R6: 100K, IMRANS_LIBRARY:R_Axial_DIN0207_L6.3mm_D2.5mm_P10.16mm_Horizontal_2, F.Cu at (234.4, 64.2)
- added R6: 100K, IMRANS_LIBRARY:R_Axial_DIN0207_L6.3mm_D2.5mm_P10.16mm_Horizontal_2, F.Cu at (83.6, 132.2)
- added R6: 100K, IMRANS_LIBRARY:R_Axial_DIN0207_L6.3mm_D2.5mm_P10.16mm_Horizontal_2, F.Cu at (234.4, 98.2)
- added R6: 100K, IMRANS_LIBRARY:R_Axial_DIN0207_L6.3mm_D2.5mm_P10.16mm_Horizontal_2, F.Cu at (83.6, 30.2)
- added R6: 100K, IMRANS_LIBRARY:R_Axial_DIN0207_L6.3mm_D2.5mm_P10.16mm_Horizontal_2, F.Cu at (159.0, 132.2)
- added R6: 100K, IMRANS_LIBRARY:R_Axial_DIN0207_L6.3mm_D2.5mm_P10.16mm_Horizontal_2, F.Cu at (159.0, 64.2)
- added R6: 100K, IMRANS_LIBRARY:R_Axial_DIN0207_L6.3mm_D2.5mm_P10.16mm_Horizontal_2, F.Cu at (234.4, 30.2)
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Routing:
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- removed copper zone on B.Cu, net Board_12-GNDREF
- removed copper zone on B.Cu, net Board_13-GNDREF
- removed copper zone on B.Cu, net Board_14-GNDREF
- removed copper zone on B.Cu, net Board_15-GNDREF
- removed copper zone on B.Cu, net Board_16-GNDREF
- removed copper zone on B.Cu, net Board_17-GNDREF
- removed copper zone on B.Cu, net Board_18-GNDREF
- removed copper zone on B.Cu, net Board_19-GNDREF
- removed copper zone on B.Cu, net Board_20-GNDREF
- removed copper zone on B.Cu, net Board_21-GNDREF
- removed copper zone on B.Cu, net Board_22-GNDREF
- removed copper zone on B.Cu, net Board_23-GNDREF
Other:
- board size 245 x 163 mm -> 225.2 x 135 mm
- board text added: "B.KORP V2.1"
- board text removed: "B."
- board text removed: "SERVE"
- board text removed: "V1.4"

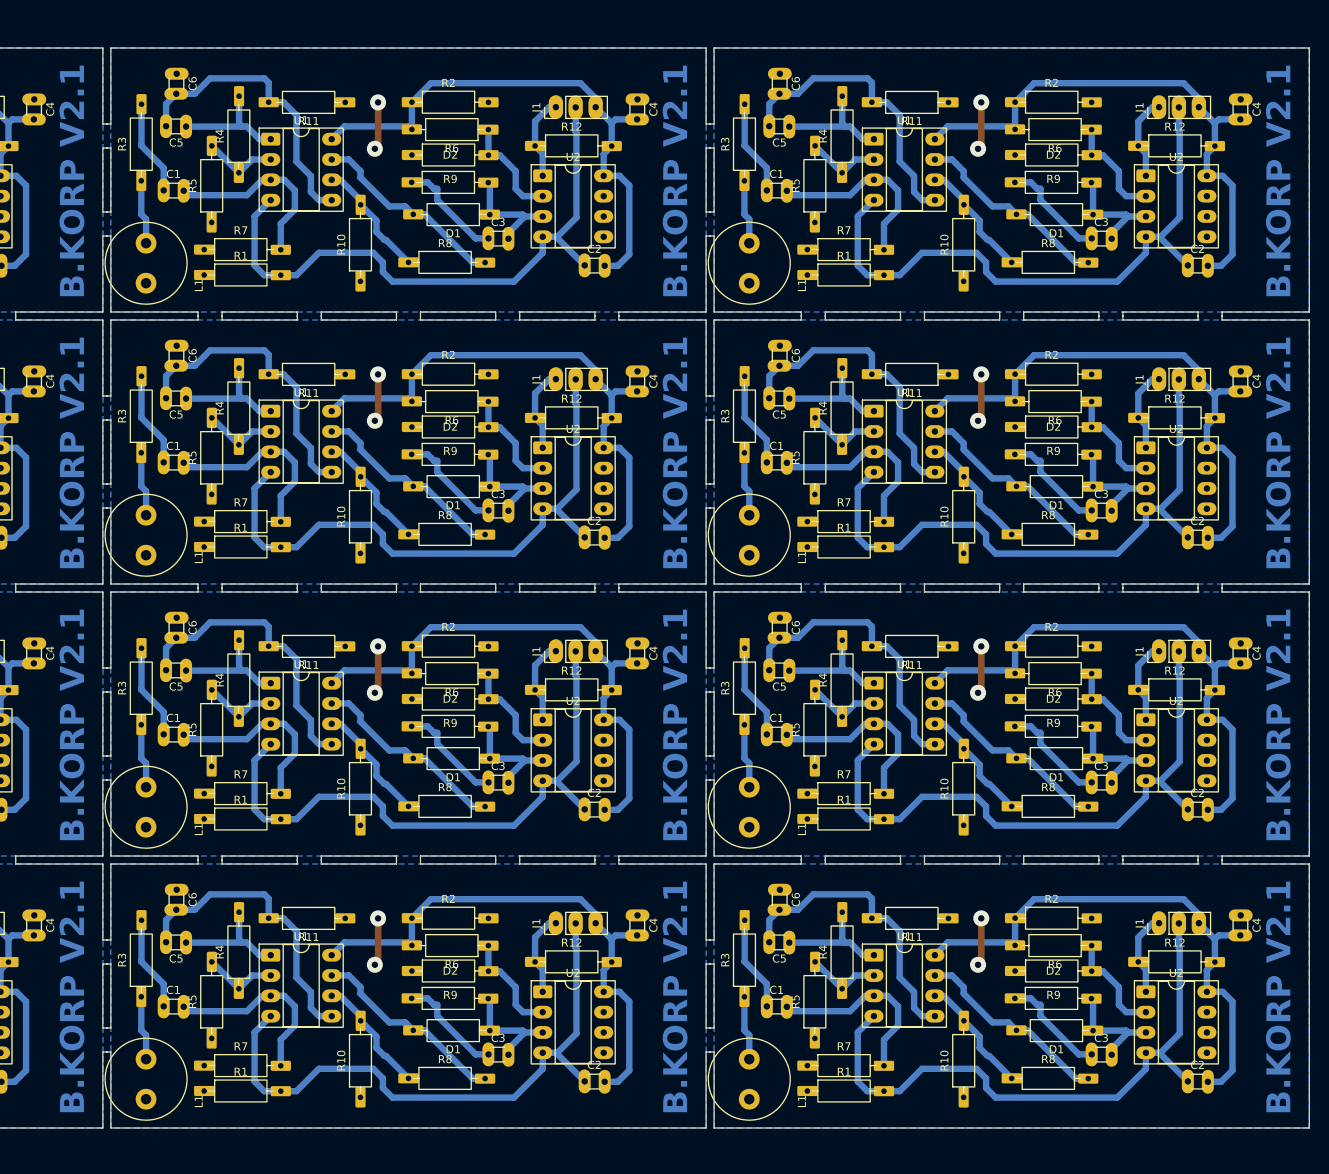
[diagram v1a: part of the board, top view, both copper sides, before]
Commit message: .
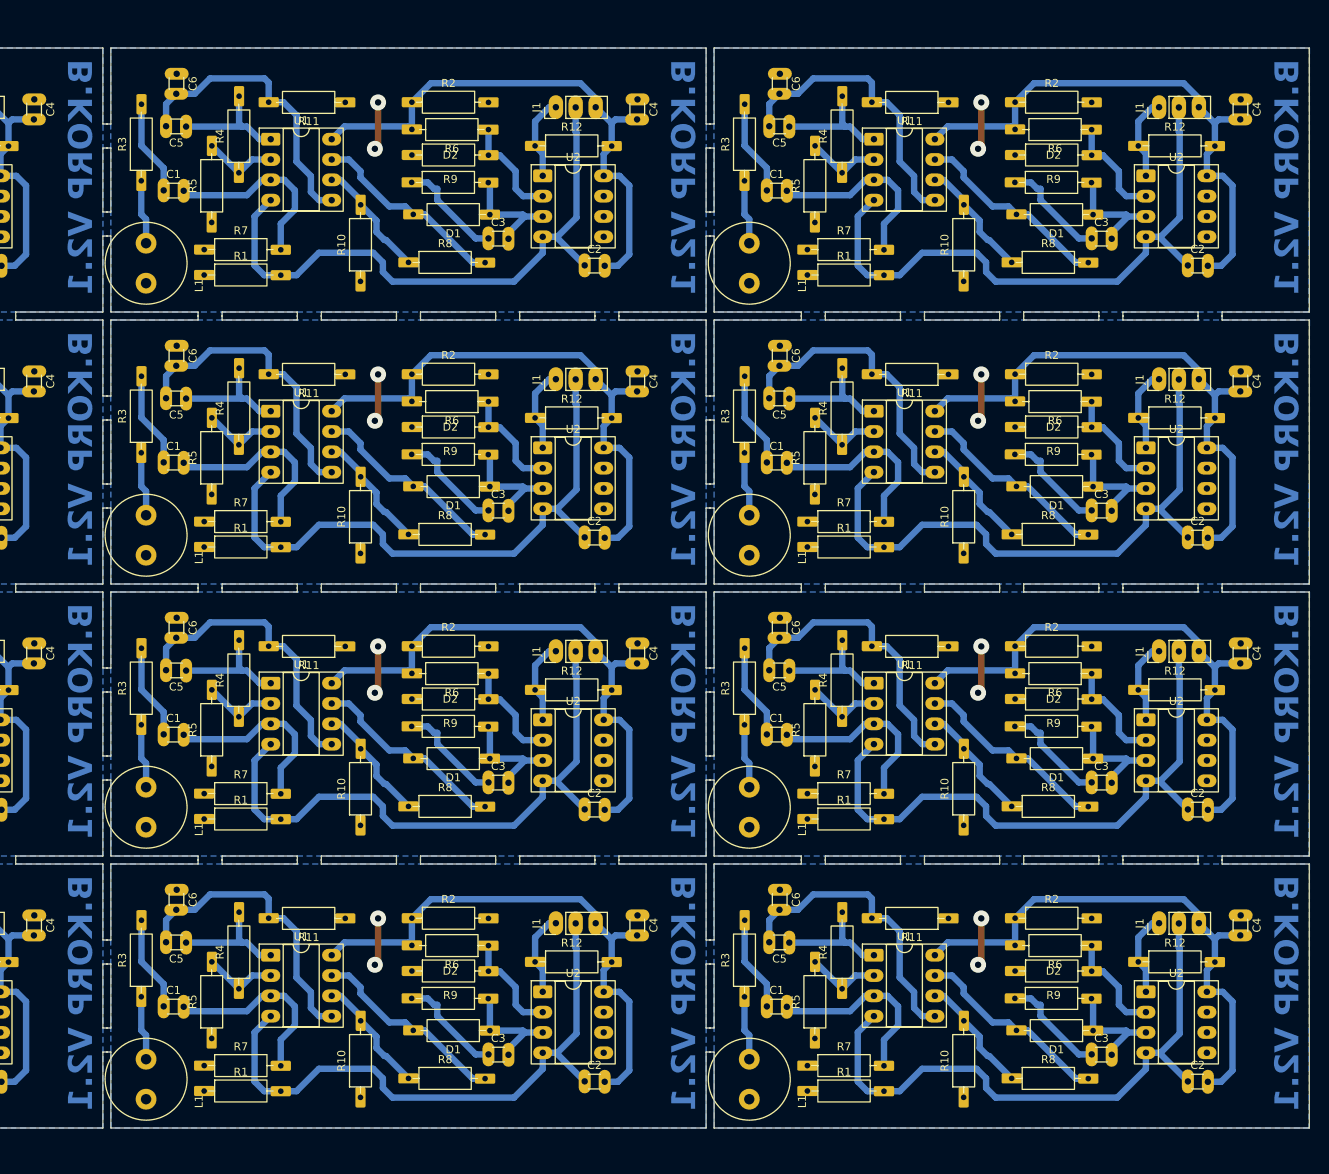
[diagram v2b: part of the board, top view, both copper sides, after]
